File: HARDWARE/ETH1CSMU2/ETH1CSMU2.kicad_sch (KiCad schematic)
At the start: 0 parts

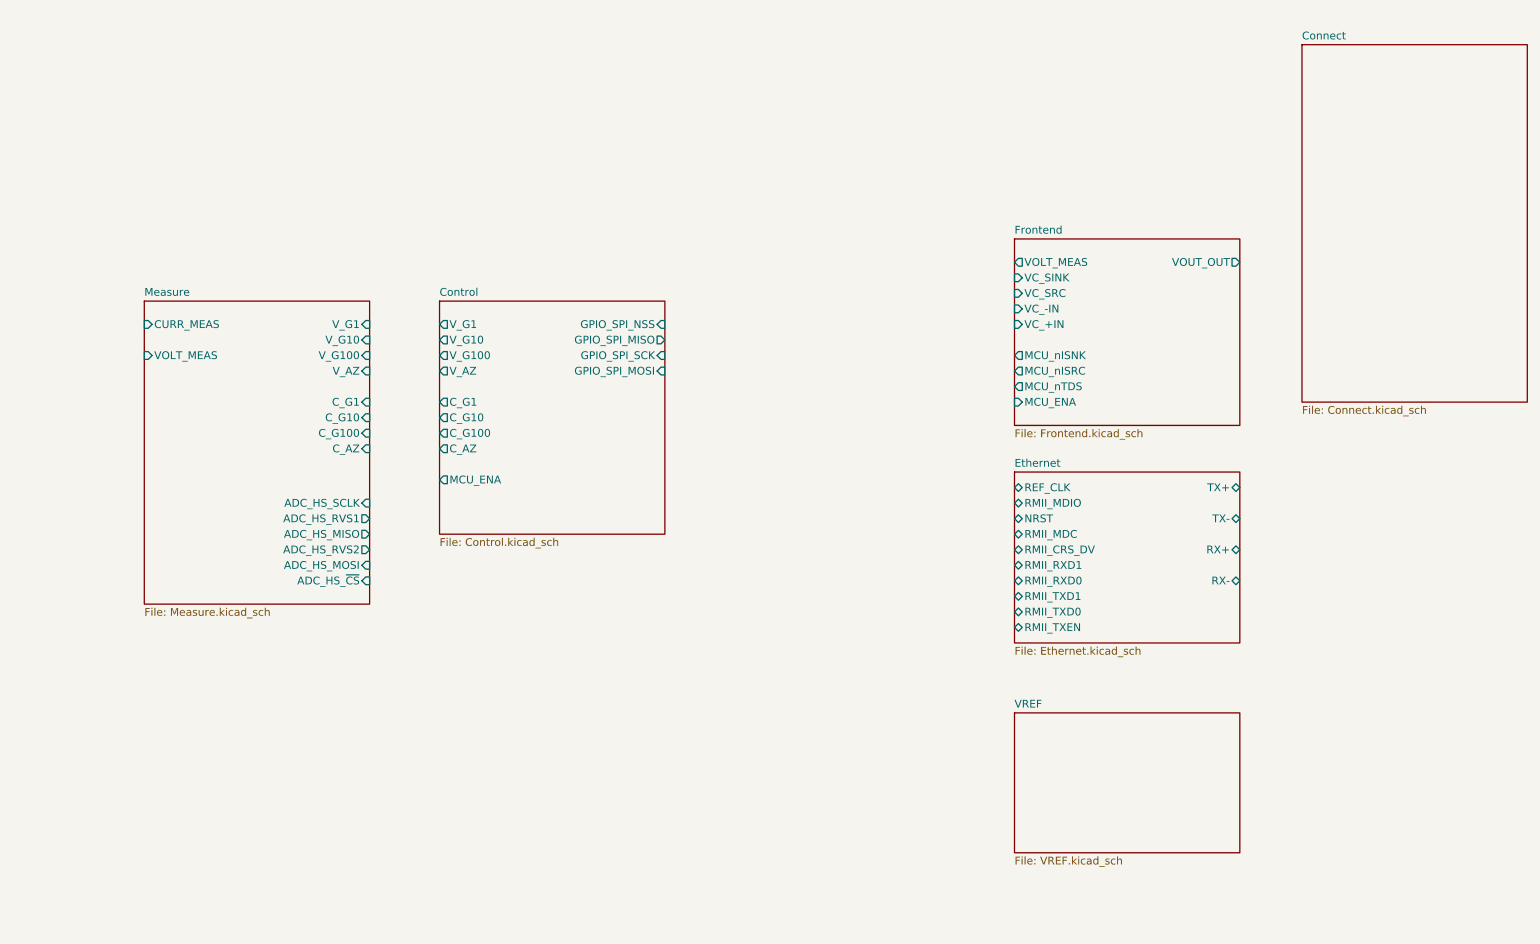
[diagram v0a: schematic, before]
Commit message: Hardware design
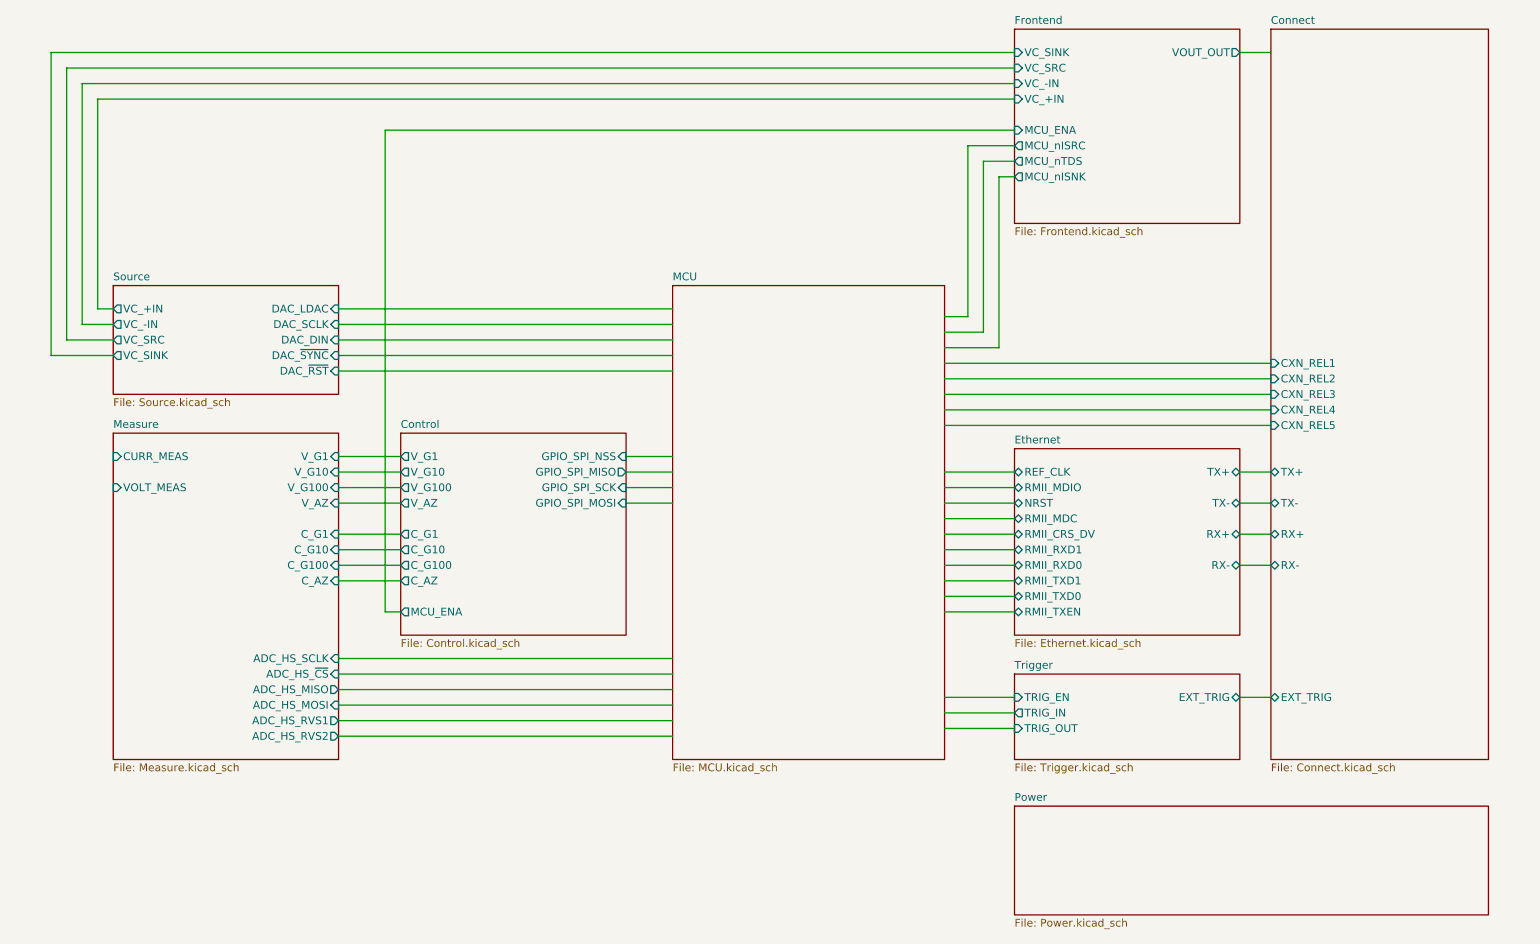
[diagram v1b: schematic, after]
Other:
- removed sheet VREF
- added sheet MCU (MCU.kicad_sch)
- added sheet Power (Power.kicad_sch)
- added sheet Source (Source.kicad_sch)
- added sheet Trigger (Trigger.kicad_sch)
- sheet Connect ports: added CXN_REL1, CXN_REL2, CXN_REL3, CXN_REL4, CXN_REL5, EXT_TRIG, RX+, RX-, TX+, TX-; removed none
- sheet Frontend ports: added none; removed VOLT_MEAS

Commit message: Hardware design
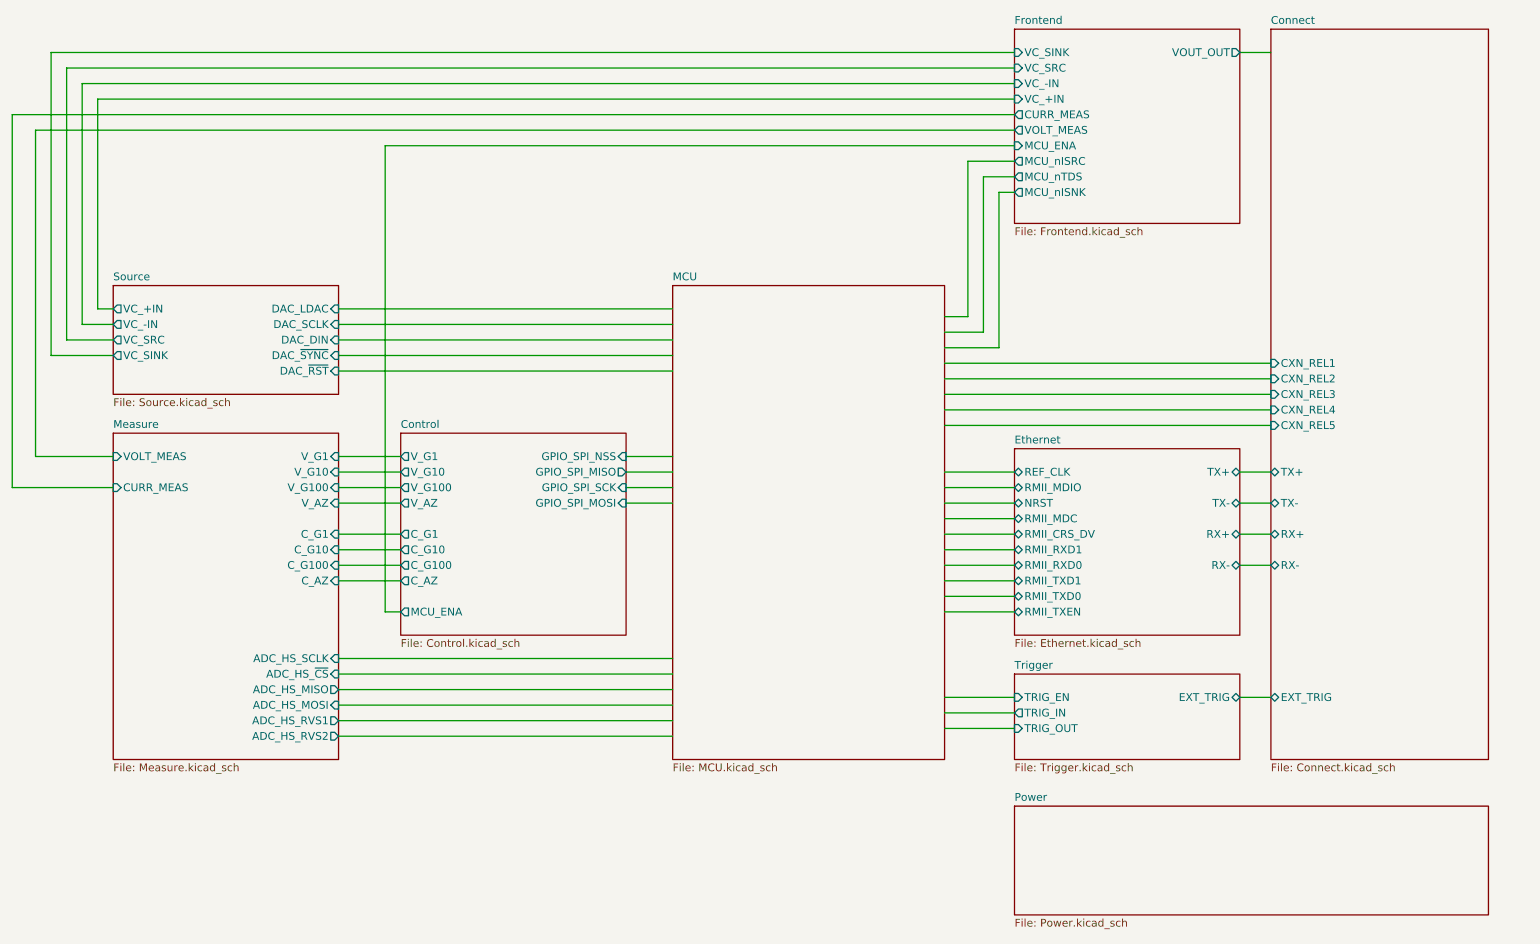
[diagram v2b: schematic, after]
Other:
- sheet Frontend ports: added CURR_MEAS, VOLT_MEAS; removed none
